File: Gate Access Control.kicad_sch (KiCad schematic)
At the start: 15 parts, among them J1 Screw_Terminal_01x02, J2 Inverter Conn., J3 Conn_01x08, SW1 SW_SPST, U1 ATmega328-P, U2 RF Receiver 433MHz, U3 IR_SENSORT, Y1 Crystal

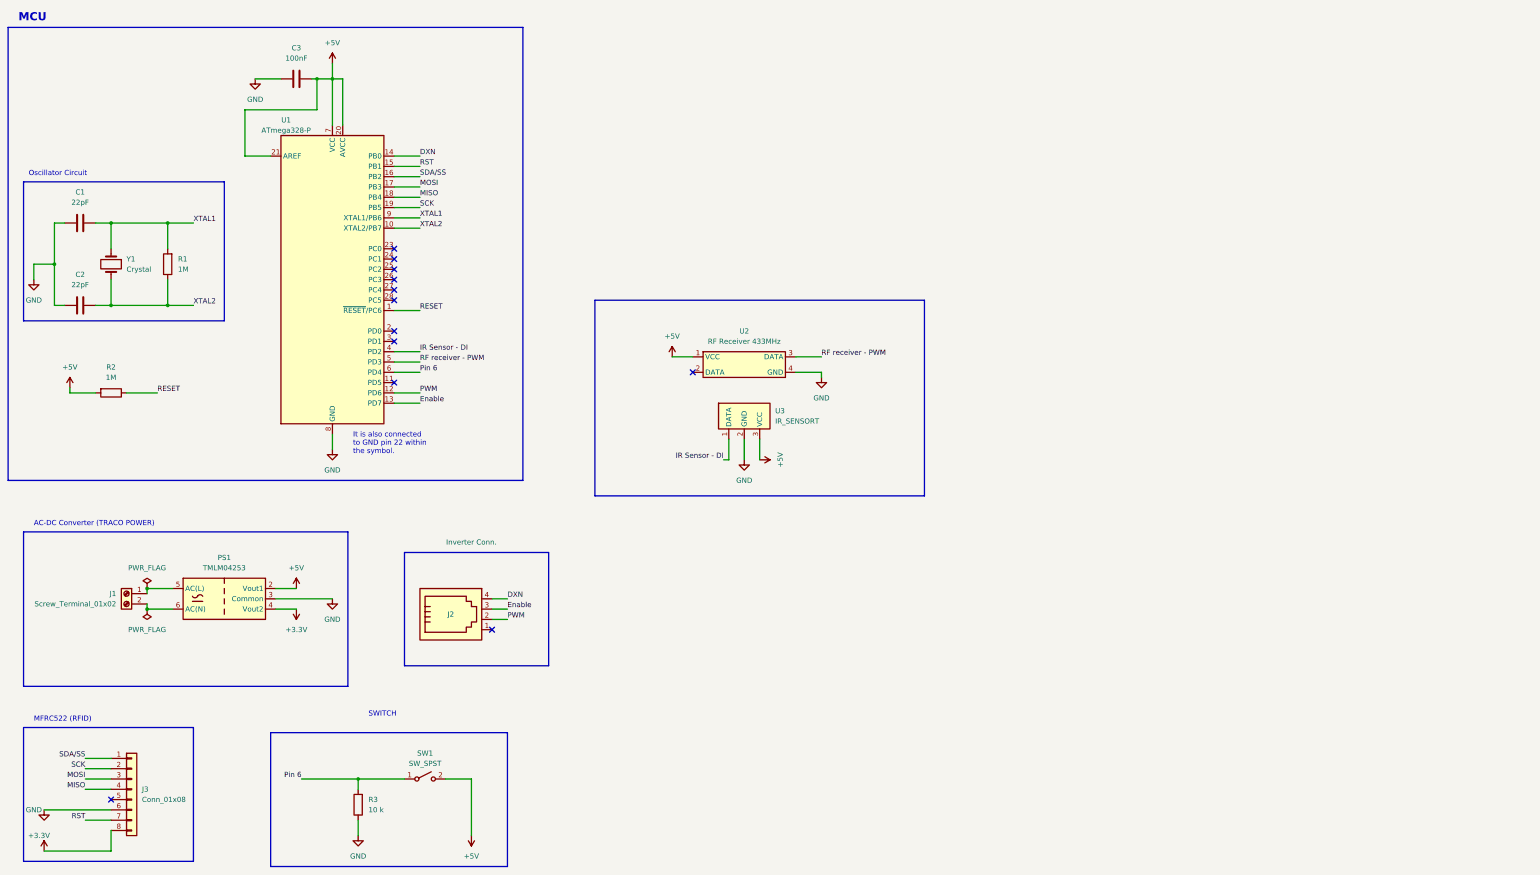
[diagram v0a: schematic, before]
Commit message: Switch and Inverter
I have updated the switch position and changed the previous connector for the inverter
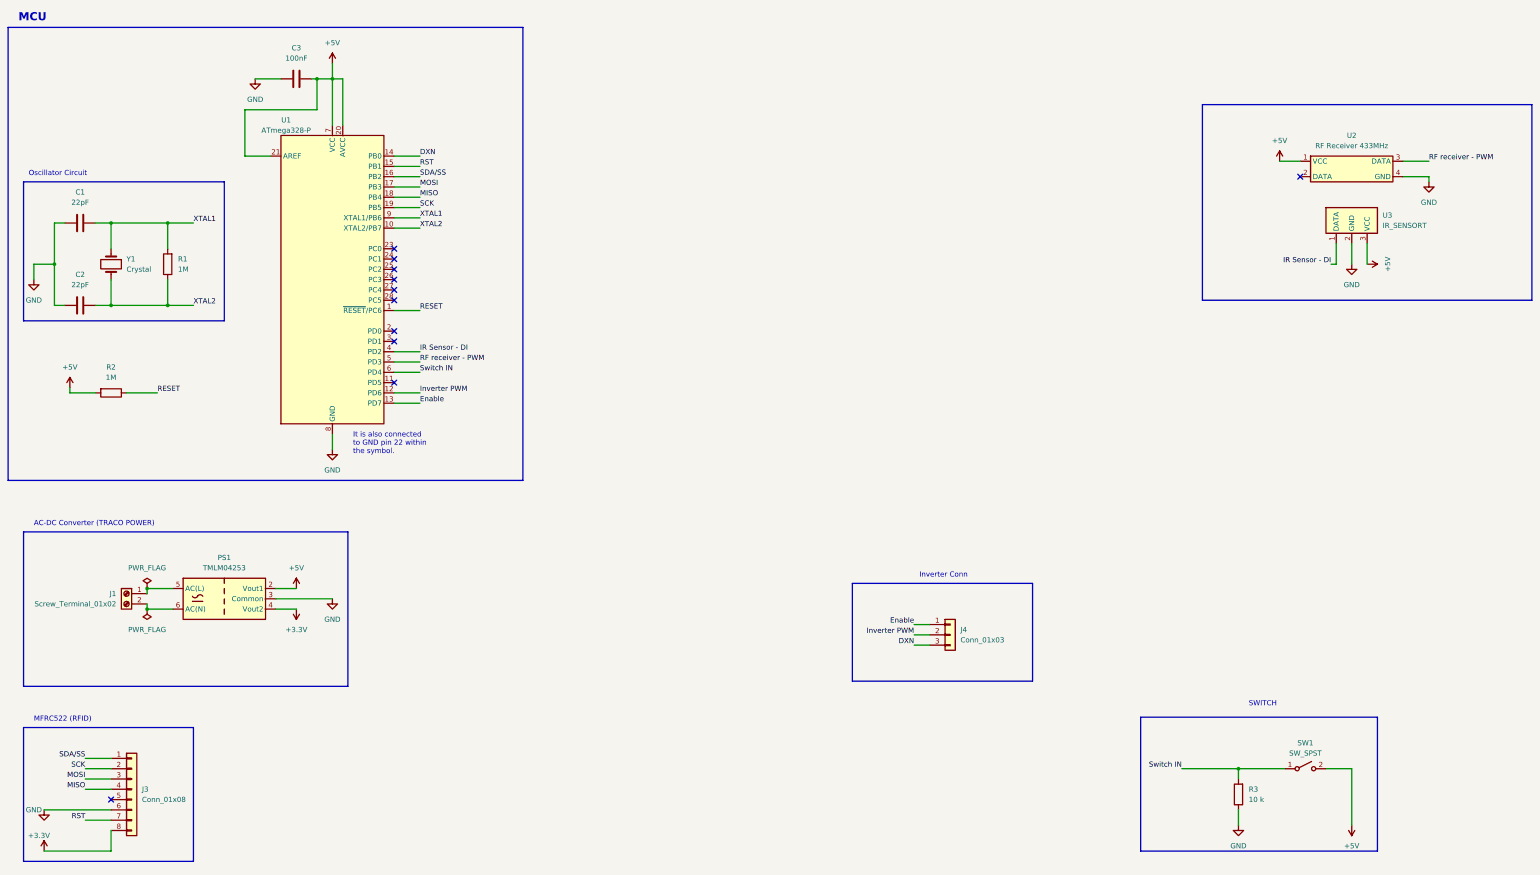
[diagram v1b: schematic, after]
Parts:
- removed J2: Inverter Conn., symbol Connector:RJ22
- added J4: Conn_01x03, symbol Connector_Generic:Conn_01x03
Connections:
- net DXN: now also J4.3 (Pin_3)
- net Enable: now also J4.1 (Pin_1)
- net PWM renamed Inverter PWM
- net Inverter PWM: now also J4.2 (Pin_2)
- net Pin 6 renamed Switch IN
- no-connect marks 12 -> 11
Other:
- note added: "Inverter Conn"
- moved on the sheet: U2, U3
